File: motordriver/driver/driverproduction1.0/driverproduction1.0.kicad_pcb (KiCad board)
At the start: 4 copper layers, 180 x 100 mm, 69 parts

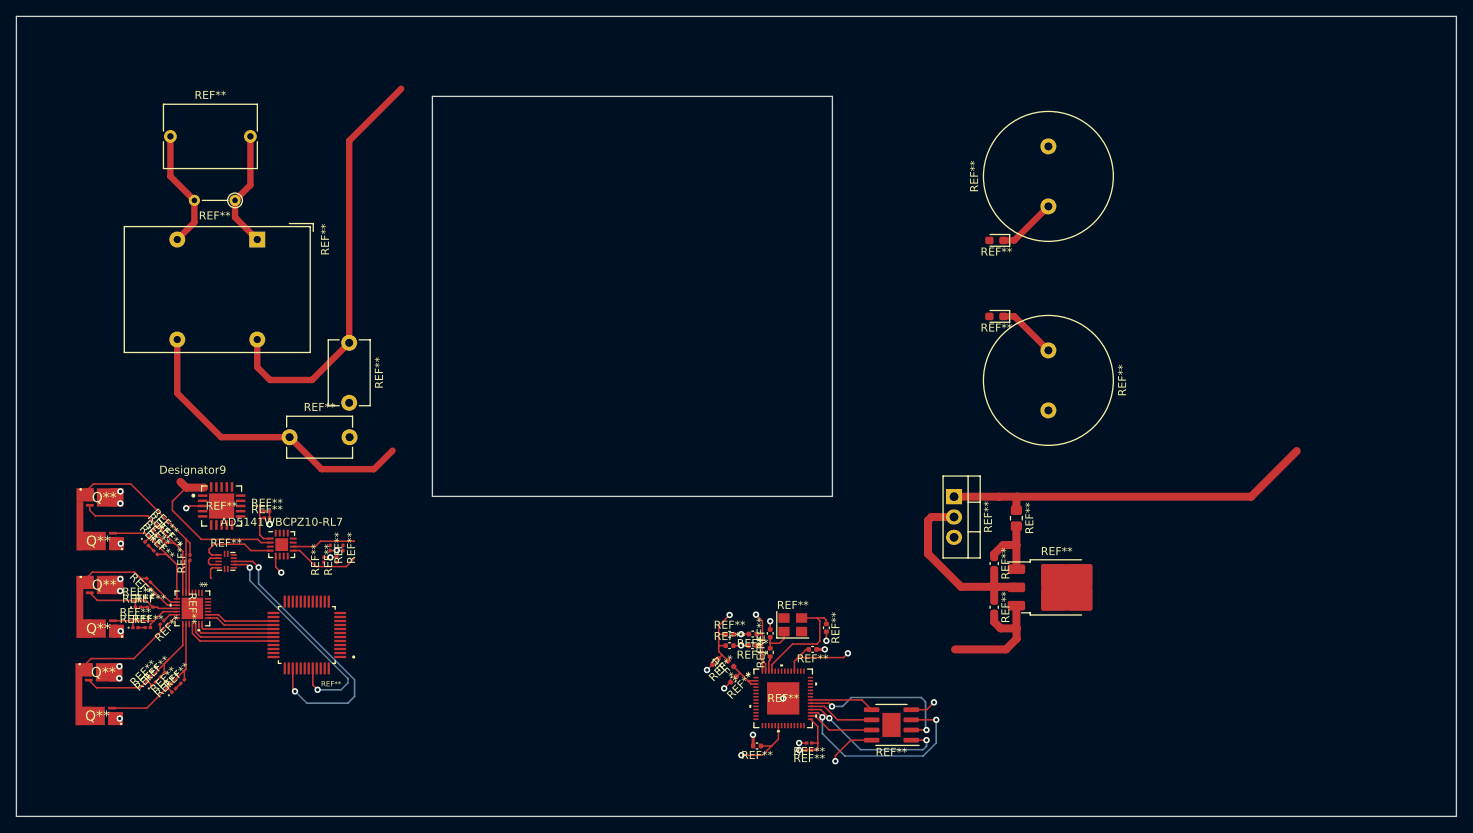
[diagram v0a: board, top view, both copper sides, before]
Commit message: larp
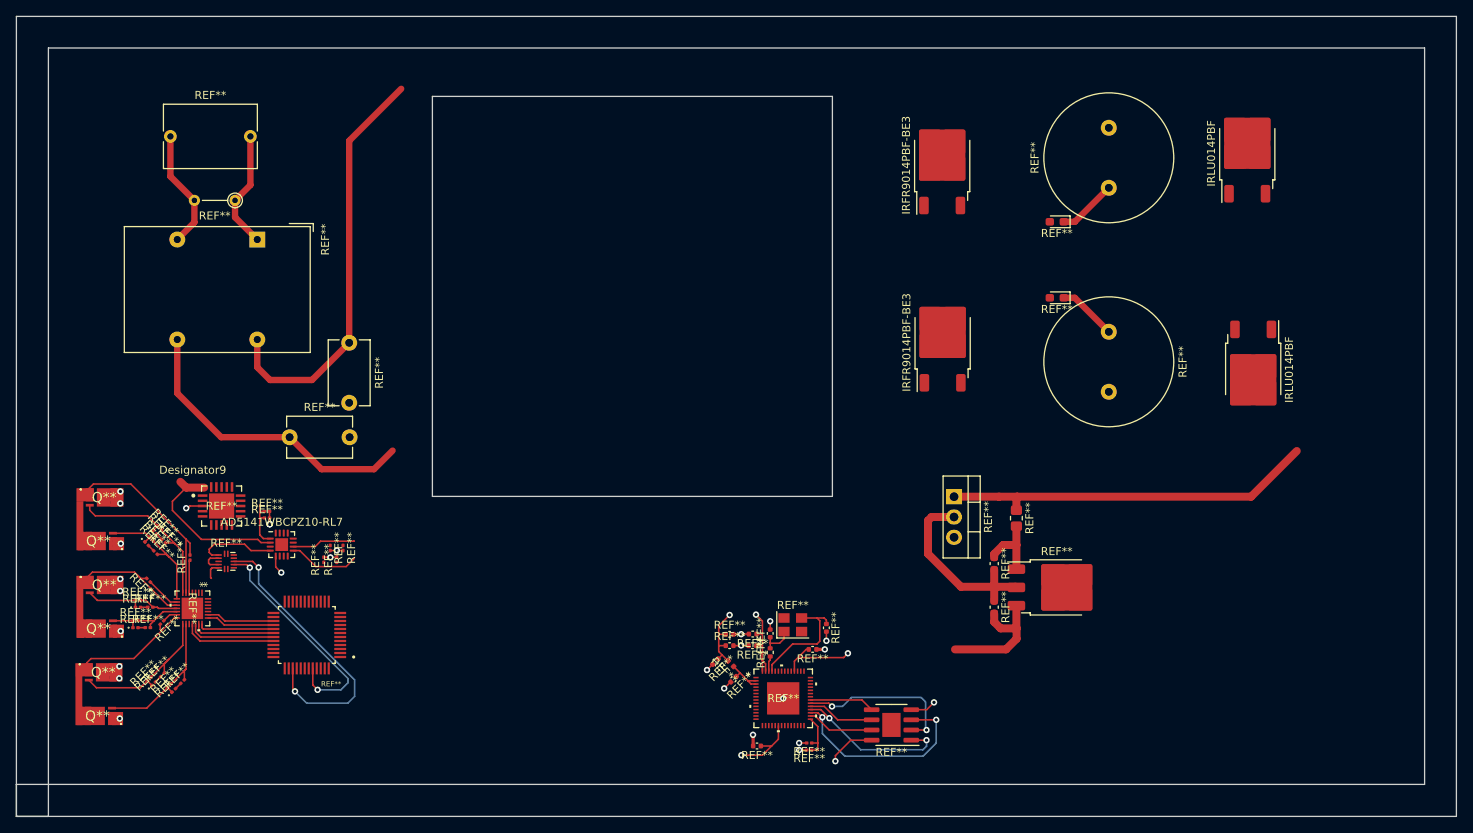
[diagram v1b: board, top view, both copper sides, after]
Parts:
- added IRFR9014PBF-BE3: TO-252-2, Package_TO_SOT_SMD:TO-252-2, F.Cu at (145.7, 38.6)
- added IRFR9014PBF-BE3: TO-252-2, Package_TO_SOT_SMD:TO-252-2, F.Cu at (145.8, 60.8)
- added IRLU014PBF: TO-252-2, Package_TO_SOT_SMD:TO-252-2, F.Cu at (183.9, 37.1)
- added IRLU014PBF: TO-252-2, Package_TO_SOT_SMD:TO-252-2, F.Cu at (184.6, 64.2)
- moved REF** 7.90 mm to (166.6, 59.4)
- moved REF** 7.90 mm to (166.6, 41.4)
- moved REF** 7.90 mm to (160.1, 45.7)
- moved REF** 7.90 mm to (160.1, 55.2)
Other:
- outline, holes or cut-outs redrawn
